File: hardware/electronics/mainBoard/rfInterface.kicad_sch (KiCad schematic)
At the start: 21 parts, among them J12 CONMHF1-SMD-T, J13 CONMHF1-SMD-T, J14 CONMHF1-SMD-T, J15 CONMHF1-SMD-T, U17 PMA2-162LNA+, U18 QCN-19D+

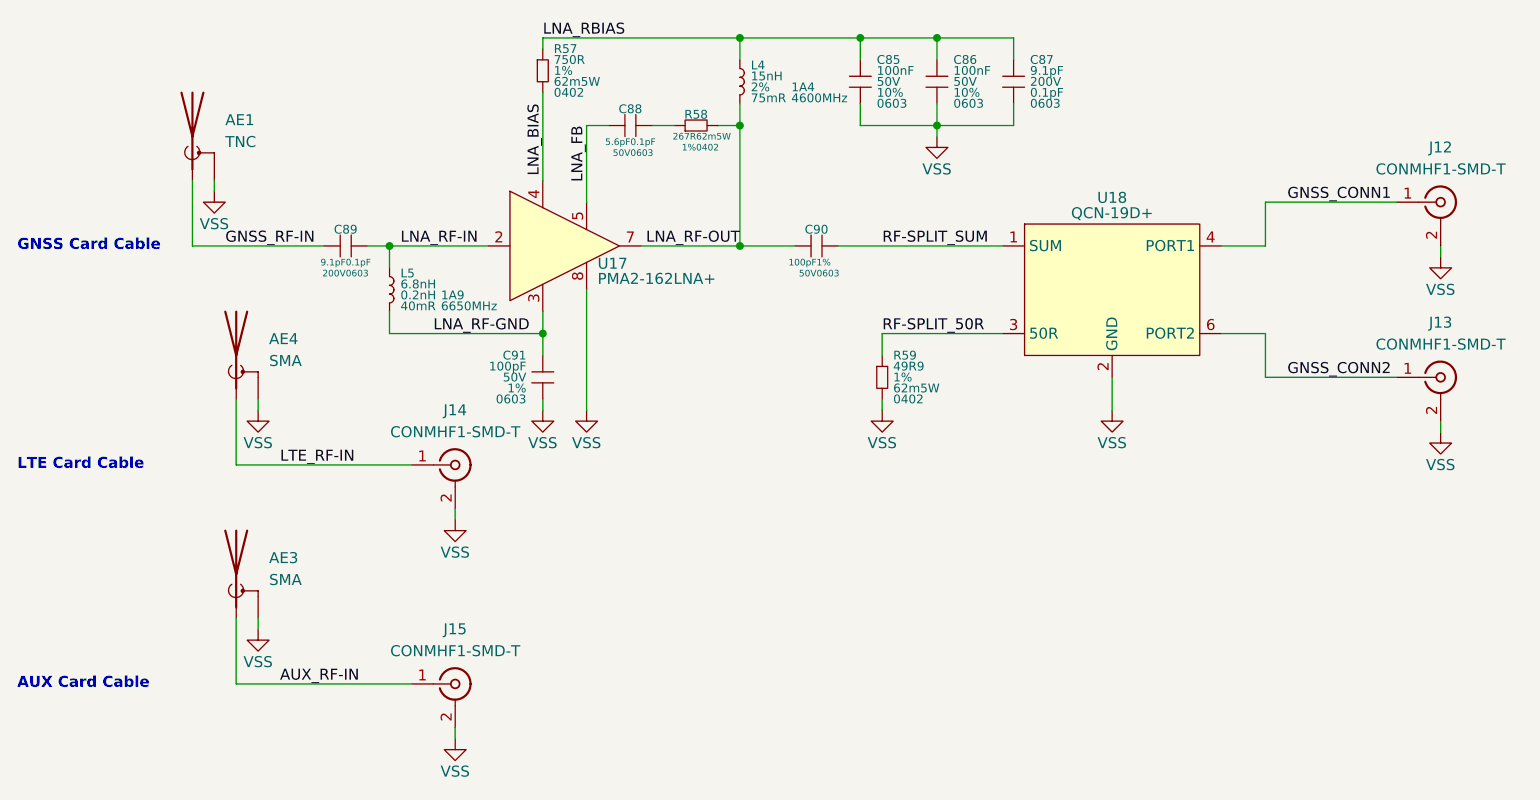
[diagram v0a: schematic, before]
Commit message: fixed power flags
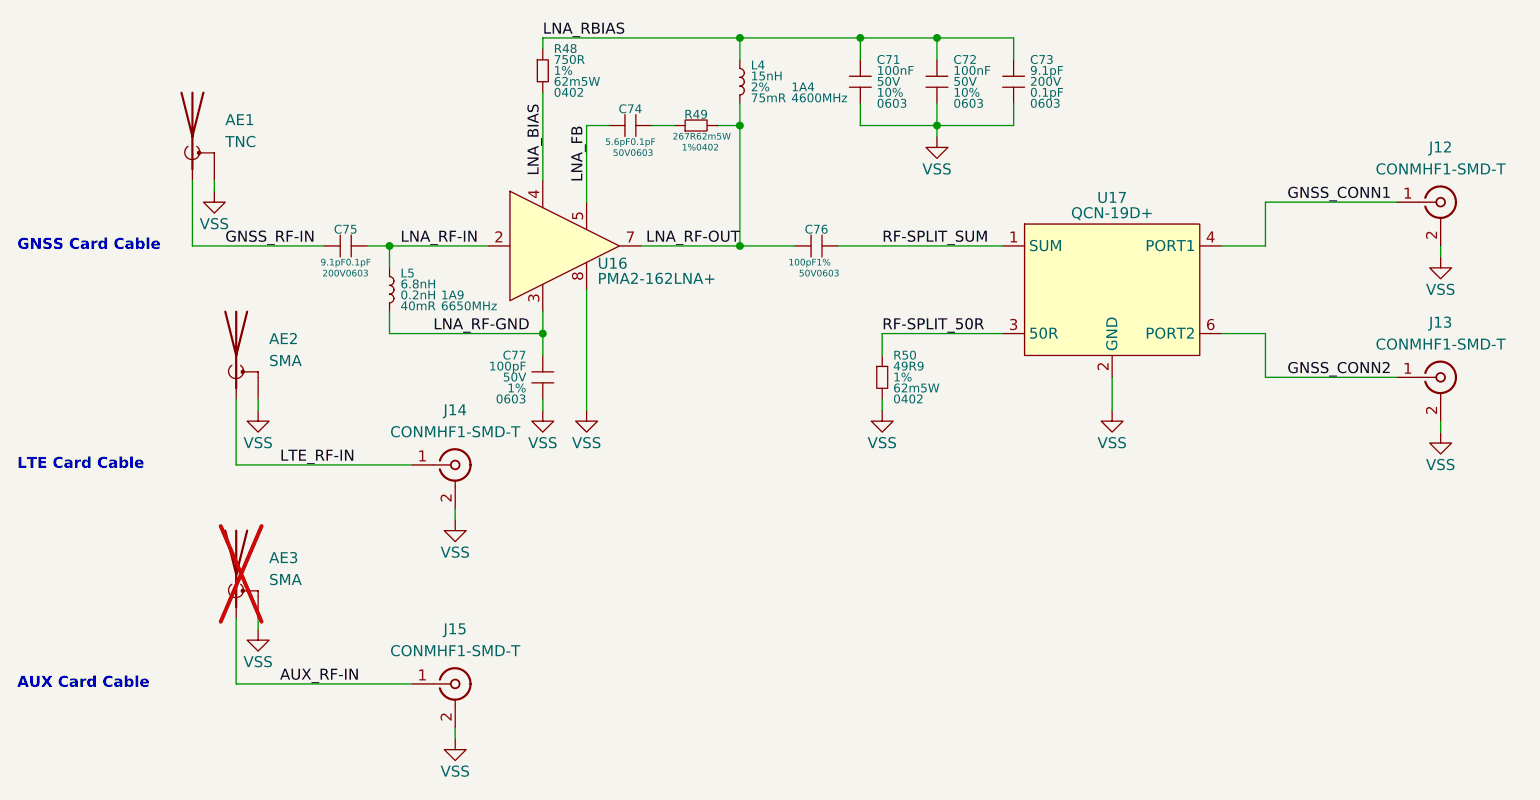
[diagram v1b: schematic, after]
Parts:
- AE3: now not fitted
- renumbered AE4 to AE2, C85 to C71, C86 to C72, C87 to C73, C88 to C74, C89 to C75, C90 to C76, C91 to C77, R57 to R48, R58 to R49, R59 to R50, U17 to U16, U18 to U17
